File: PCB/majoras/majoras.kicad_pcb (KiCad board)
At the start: 2 copper layers, 13 x 6.5 mm, 13 parts

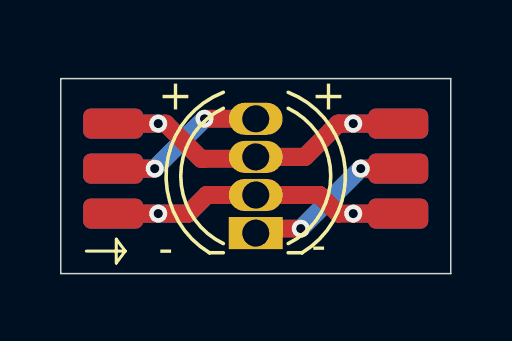
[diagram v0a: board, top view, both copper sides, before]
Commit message: Updated fabrication files
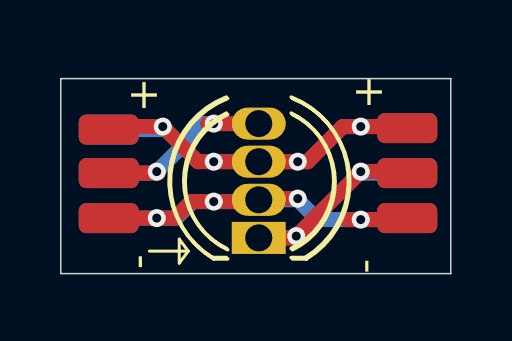
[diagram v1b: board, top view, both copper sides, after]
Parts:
- moved REF** 0.34 mm to (154.8, 91.9) (x2)
- moved REF** 0.34 mm to (154.8, 88.9) (x2)
- moved REF** 0.34 mm to (154.8, 90.4) (x2)
- moved REF** 0.25 mm to (144.8, 89.0) (x2)
- moved REF** 0.21 mm to (144.8, 90.4) (x2)
- moved REF** 0.21 mm to (144.8, 91.9) (x2)
- moved D1 0.19 mm to (149.8, 92.6)
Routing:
- net DIN: track 6.82 -> 9.03 mm
- net VDD: track 17.2 -> 19.1 mm, vias 2 -> 4
- net GND: track 16.5 -> 18.4 mm, vias 2 -> 4
- net DOUT: track 6.89 -> 8.58 mm
